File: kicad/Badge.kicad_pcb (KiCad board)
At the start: 2 copper layers, 109 x 57.4 mm, 26 parts, among them SW1 SW_SPST, U1 LMC555xM

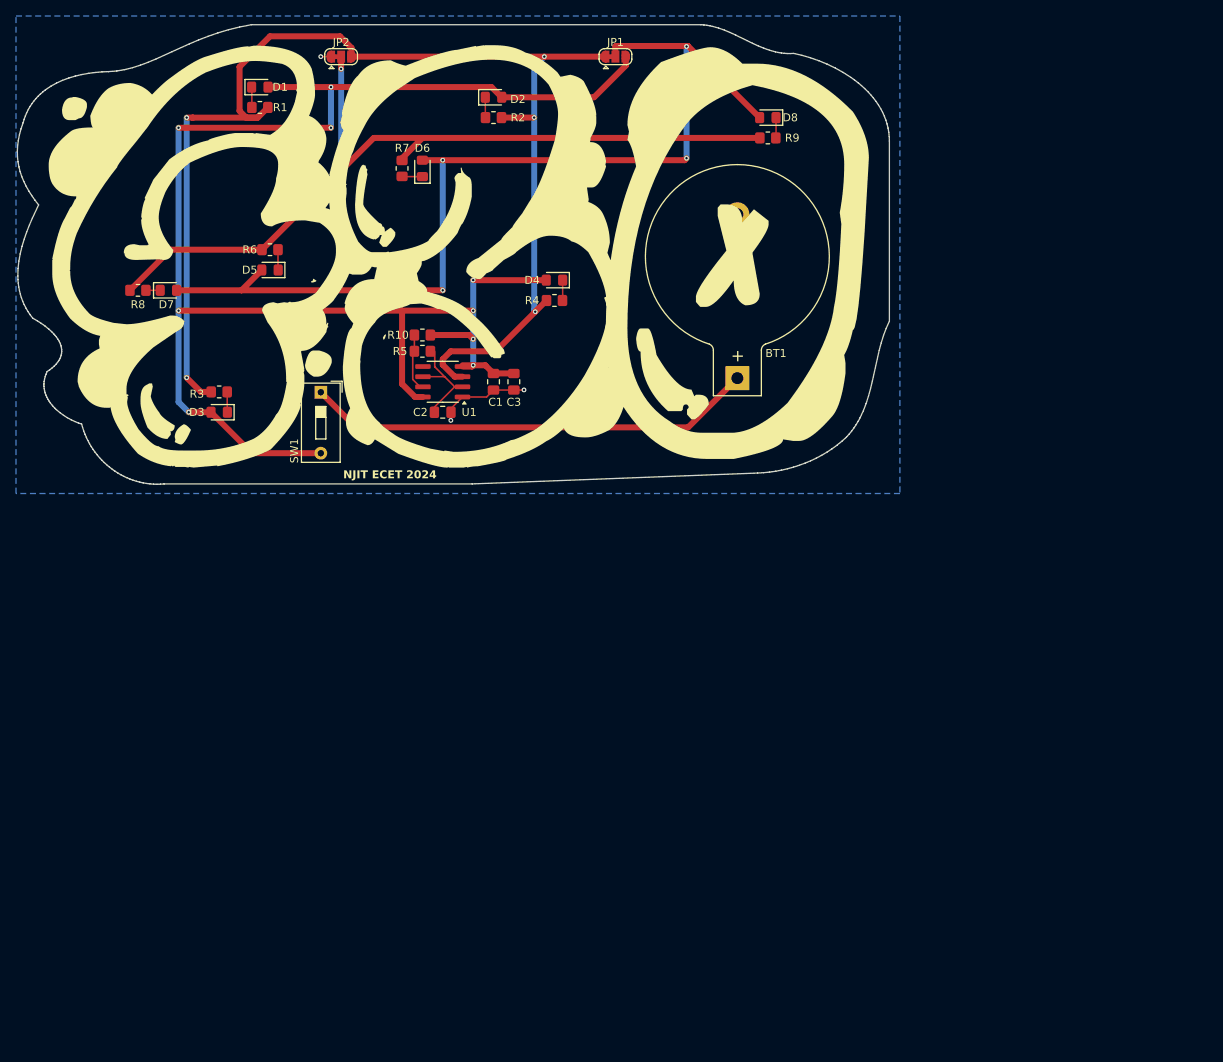
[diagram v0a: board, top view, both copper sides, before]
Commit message: 230 refactor
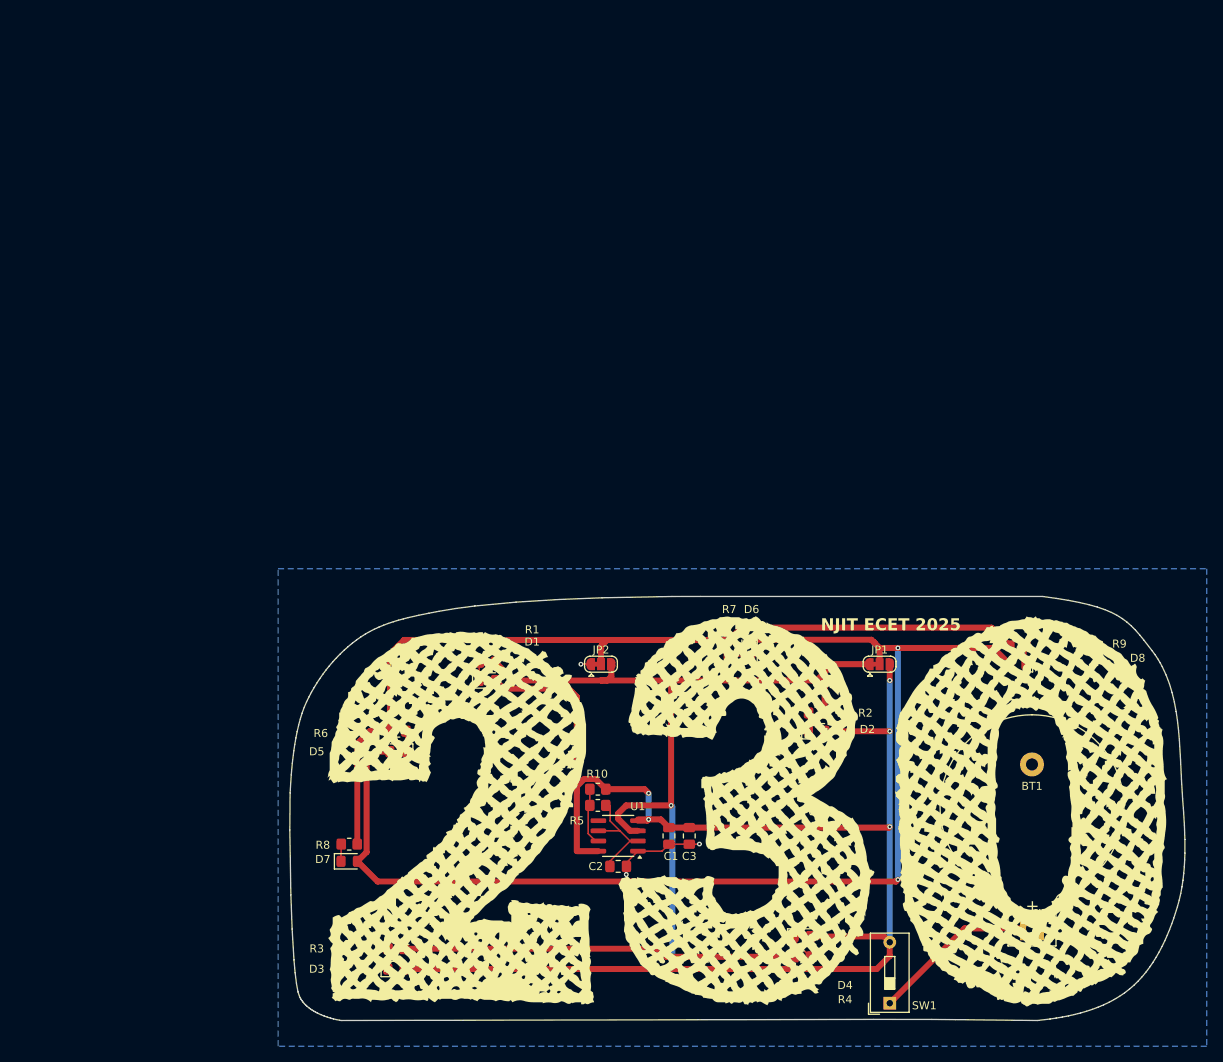
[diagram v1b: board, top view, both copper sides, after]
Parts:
- moved SW1 104.4 mm to (146.1, 151.3), turned to 90 degrees
- moved D2 88.9 mm to (136.9, 117.3)
- moved D4 87.7 mm to (135.1, 143.0), turned to 0 degrees
- moved R4 87.7 mm to (135.1, 145.5)
- moved R2 84.7 mm to (136.9, 115.1)
- moved JP1 82.8 mm to (144.8, 109.0)
- moved JP2 82.6 mm to (110.0, 109.0)
- moved D1 79.4 mm to (95.8, 111.0)
- moved BT1 78.0 mm to (163.8, 142.0)
- moved D8 75.1 mm to (162.1, 109.0)
- moved R1 75.0 mm to (95.8, 108.7)
- moved D7 74.9 mm to (78.5, 133.6)
- moved R8 74.1 mm to (78.5, 131.5), turned to 0 degrees
- moved D3 73.0 mm to (84.3, 147.1), turned to 0 degrees
- moved R3 73.0 mm to (84.3, 144.5), turned to 0 degrees
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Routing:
- net /BAT: track 56.4 -> 21.7 mm
- net /PULSE2H: track 123.2 -> 150.2 mm, vias 4 -> 2
- net VCC: track 209.7 -> 196.6 mm, vias 9 -> 5
- net /PULSE: track 160.4 -> 151.4 mm, vias 5 -> 2
- net /PULSE2L: track 104.7 -> 110.1 mm, vias 2 -> 0
- net Net-(D4-K): track 2.59 -> 3.41 mm
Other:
- board size 109 x 57.4 mm -> 111.9 x 53 mm
- board text added: "NJIT ECET 2025"
- board text removed: "NJIT ECET 2024"
